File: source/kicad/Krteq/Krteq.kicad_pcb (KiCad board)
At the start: 2 copper layers, 228.6 x 114.3 mm, 199 parts, among them J71 OLED 128x32, SW1 Switch, SW10 Switch, SW11 Switch, SW12 Switch, SW13 Switch, SW14 Switch, SW15 Switch, SW16 Switch, SW17 Switch, SW18 Switch, SW19 Switch, SW2 Switch, SW20 Switch, SW21 Switch, SW22 Switch, SW23 Switch, SW24 Switch, SW25 Switch, SW26 Switch, SW27 Switch, SW28 Switch, SW29 Switch, SW3 Switch, SW30 Switch, SW31 Switch, SW32 Switch, SW33 Switch, SW34 Switch, SW35 Switch, SW36 Switch, SW37 Switch, SW38 Switch, SW39 Switch, SW4 Switch, SW40 Switch, SW41 Switch, SW42 Switch, SW43 Switch, SW44 Switch, SW45 Switch, SW46 Switch, SW47 Switch, SW48 Switch, SW49 Switch, SW5 Switch, SW50 Switch, SW51 Switch, SW52 Switch, SW53 Switch, SW54 Switch, SW55 Switch, SW56 Switch, SW57 Switch, SW58 Switch, SW59 Switch, SW6 Switch, SW60 Switch, SW61 Switch, SW7 Switch, SW8 Switch, SW9 Switch, U71 IS31FL3733-QF

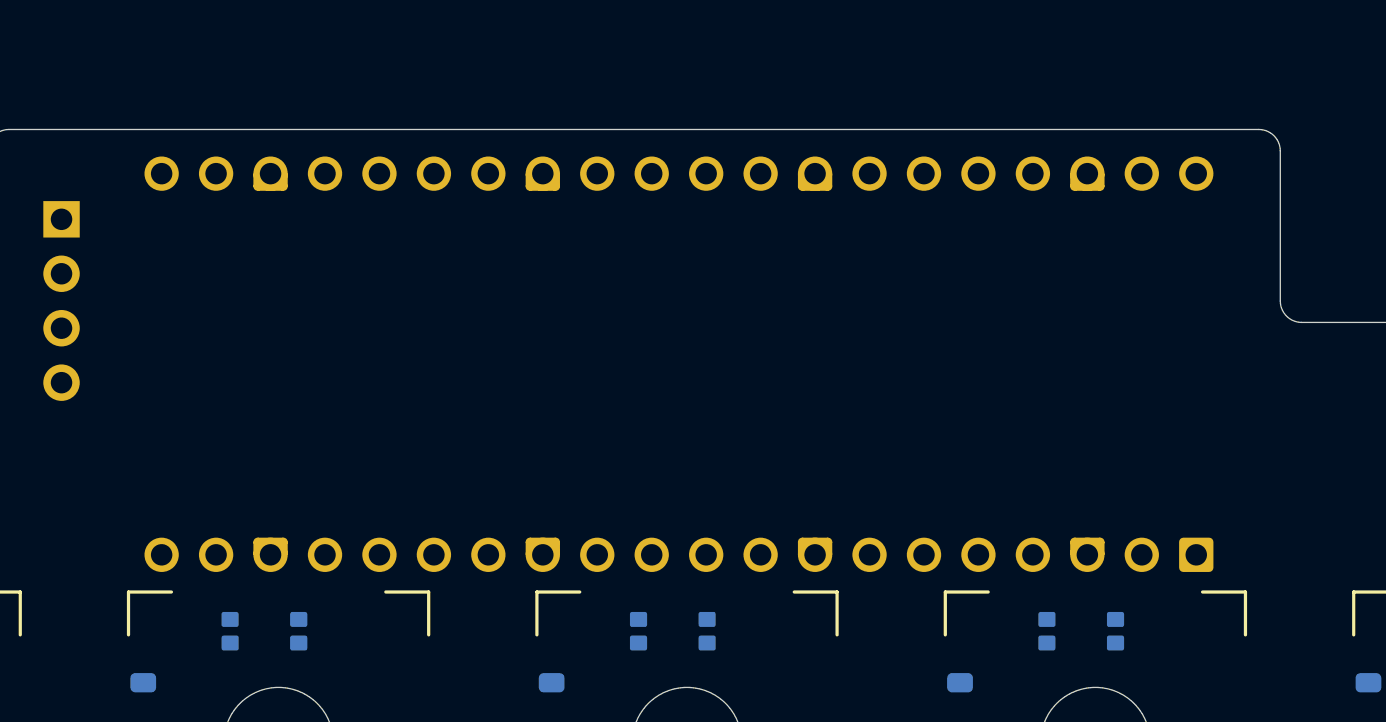
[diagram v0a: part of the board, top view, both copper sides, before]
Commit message: update
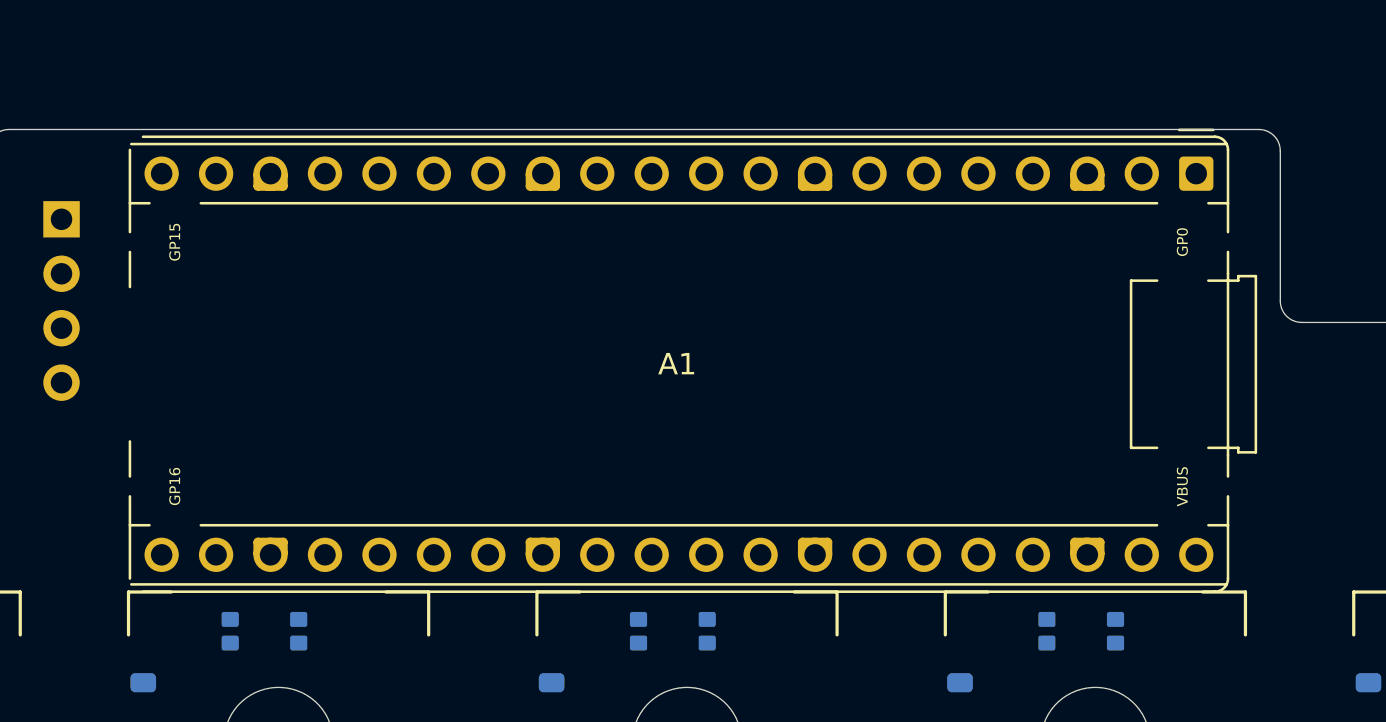
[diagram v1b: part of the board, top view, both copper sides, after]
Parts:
- A1: moved to F.Cu
- turned A1 to -90 degrees
